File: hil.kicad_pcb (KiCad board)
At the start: 2 copper layers, 184.8 x 55.9 mm, 76 parts, among them J1 5V In, J10 GND1, J11 GND3, J12 Programming Connector, J13 PPS IO, J14 Power Input, J15 PPS IO, J16 Power Input, J17 PPS IO, J18 Power Input, J19 PPS IO, J2 USB_B, J20 Power Input, J21 PPS IO, J22 Power Input, J23 PPS IO, J24 Power Input, J25 PPS IO, J26 Power Input, J27 PPS IO, J28 Power Input, J29 PPS IO, J3 IO A, J30 Power Input, J31 PPS IO, J32 Power Input, J33 GND2, J34 5V1, J35 5V2, J36 GND4, J37 GND5, J38 GND6, J39 5V3, J4 IO B, J40 5V4, J5 CAN B, J6 GND, J7 CAN A, J8 I2C, J9 3V3, U1 MCP2515, U2 AZ1117-3.3, U3 MCP2562, U4 PIC24FJ128GC010, Y1 12 MHz, Y2 48 MHz DNP

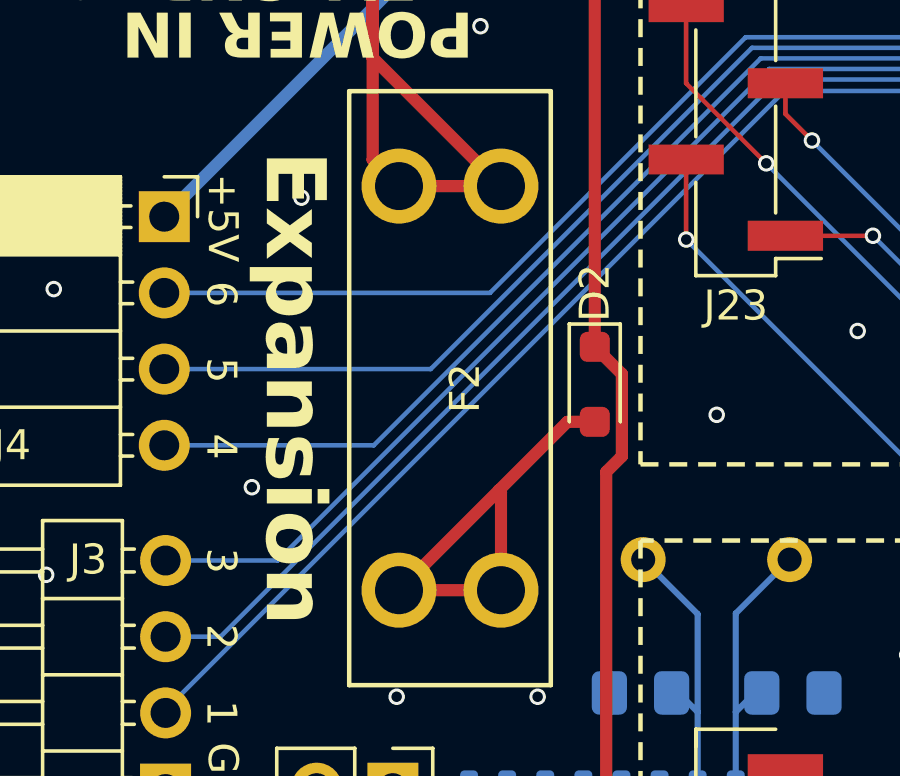
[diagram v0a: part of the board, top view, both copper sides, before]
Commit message: Address review comments
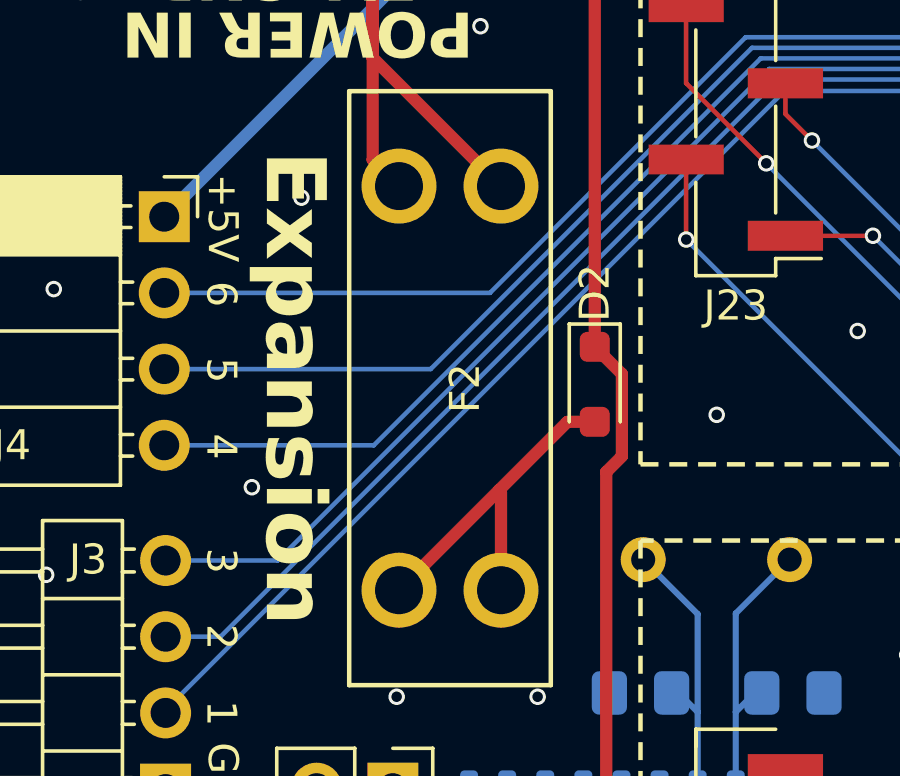
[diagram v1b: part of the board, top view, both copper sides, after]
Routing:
- net Net-(J1-Pin_1): track 30.2 -> 26.8 mm
- net Net-(D2-A): track 15.6 -> 12.2 mm
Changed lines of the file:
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@@
   (gr_line (start 199.39 154.305) (end 207.645 154.305)
     (stroke (width 0.15) (type dash)) (layer "F.SilkS"))
+  (gr_circle (center 90.17 150.495) (end 94.92 150.495)
+    (stroke (width 0.15) (type default)) (fill none) (layer "Dwgs.User"))
   (gr_line (start 216.535 127.635) (end 216.535 127.635)
     (stroke (width 0.15) (type dot)) (layer "Dwgs.User"))
+  (gr_circle (center 90.17 104.775) (end 94.92 104.775)
+    (stroke (width 0.15) (type default)) (fill none) (layer "Dwgs.User"))
+  (gr_circle (center 204.47 150.495) (end 209.22 150.495)
+    (stroke (width 0.15) (type default)) (fill none) (layer "Dwgs.User"))
+  (gr_circle (center 204.47 104.775) (end 209.22 104.775)
+    (stroke (width 0.15) (type default)) (fill none) (layer "Dwgs.User"))
   (gr_line (start 38.1 127.635) (end 242.57 127.635)
     (stroke (width 0.15) (type dot)) (layer "Dwgs.User"))
@@
   (segment (start 65.835 127.303) (end 65.7635 127.2315) (width 0.4064) (layer "F.Cu") (net 10))
   (segment (start 62.435 130.56) (end 65.7635 127.2315) (width 0.4064) (layer "F.Cu") (net 10))
-  (segment (start 62.435 130.56) (end 65.835 130.56) (width 0.4064) (layer "F.Cu") (net 10))
   (segment (start 65.7635 127.2315) (end 68.047 124.948) (width 0.4064) (layer "F.Cu") (net 10))
   (segment (start 68.047 124.948) (end 68.961 124.948) (width 0.4064) (layer "F.Cu") (net 10))
@@
   (segment (start 61.555 104.775) (end 61.555 116.21) (width 0.4064) (layer "F.Cu") (net 12))
   (segment (start 61.555 116.21) (end 62.435 117.09) (width 0.4064) (layer "F.Cu") (net 12))
-  (segment (start 62.435 117.09) (end 65.835 117.09) (width 0.4064) (layer "F.Cu") (net 12))
   (segment (start 61.555 112.81) (end 65.835 117.09) (width 0.4064) (layer "F.Cu") (net 12))
   (segment (start 61.555 104.775) (end 61.555 112.81) (width 0.4064) (layer "F.Cu") (net 12))
